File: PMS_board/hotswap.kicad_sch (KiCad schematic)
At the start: 28 parts, among them Q11 Q_NMOS_GDS, Q12 Q_NMOS_GDS, Q3 Q_NMOS_GDS, Q4 Q_NMOS_GDS, U12 LM74800QDRRRQ1, U7 LM74800QDRRRQ1

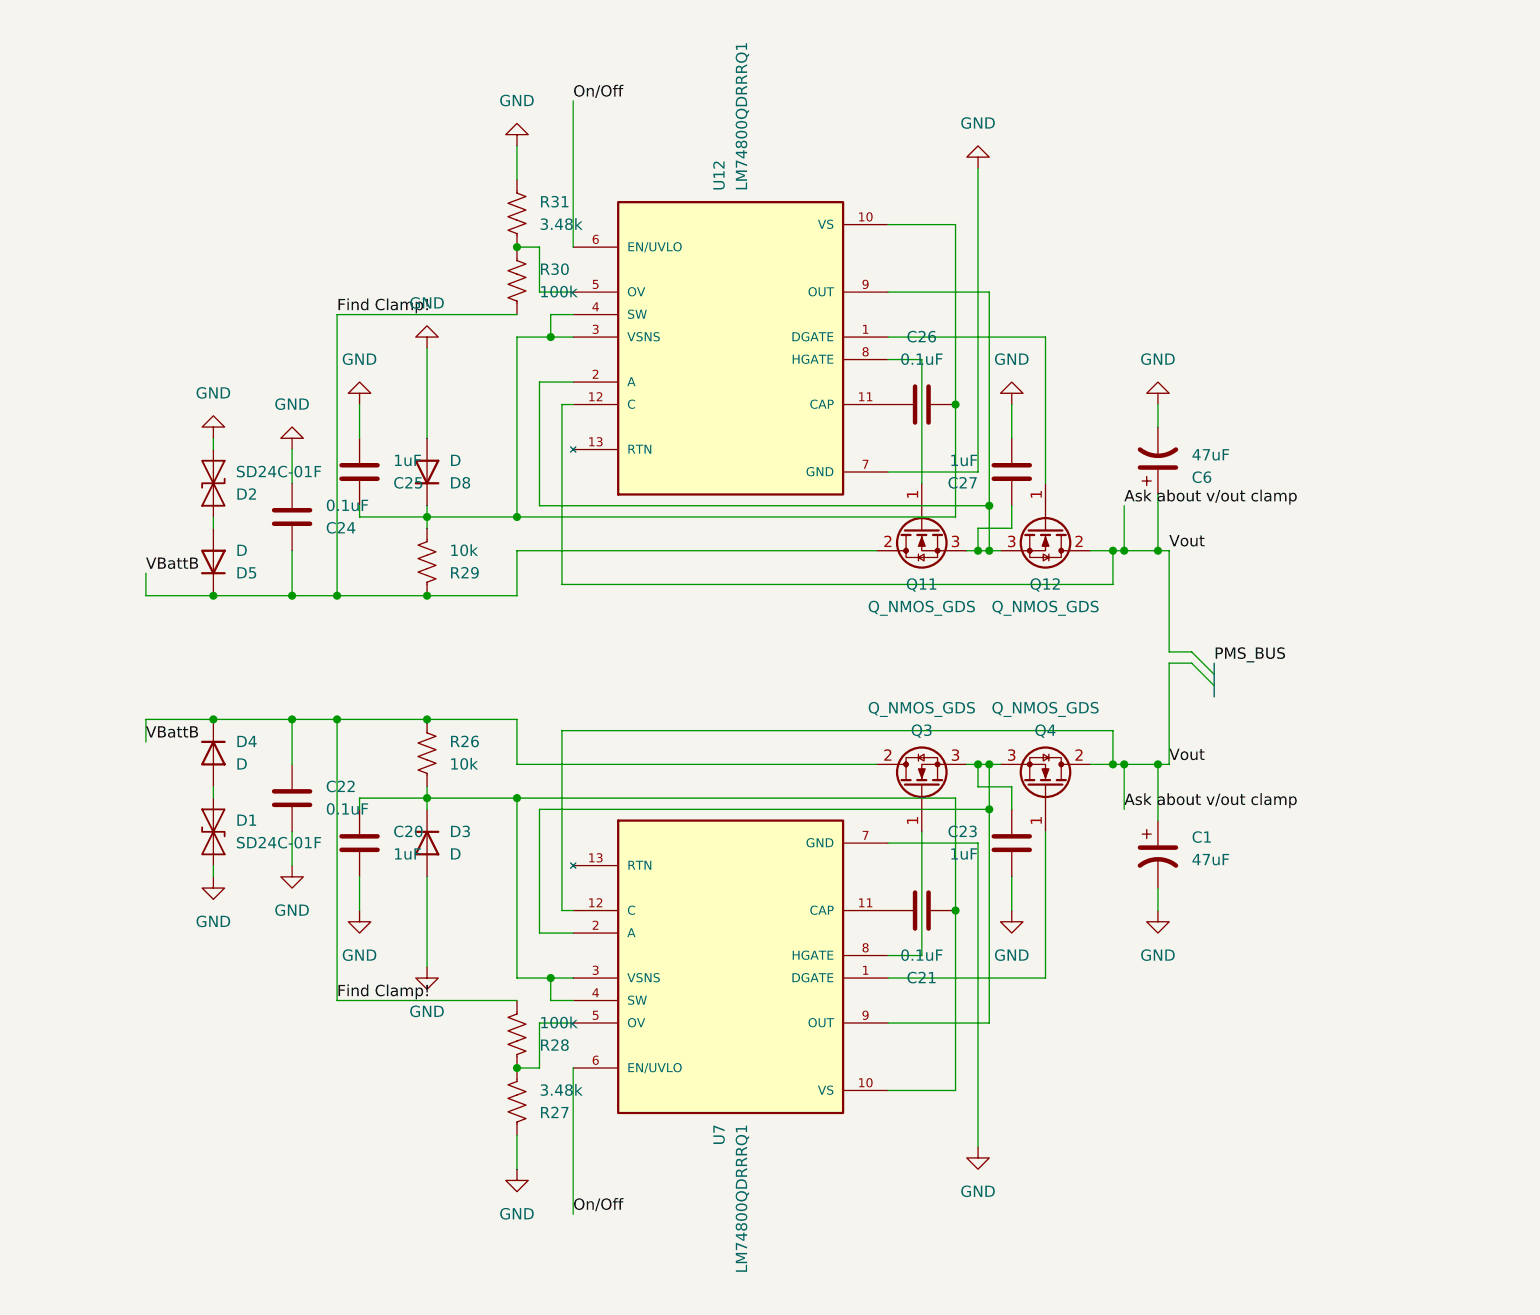
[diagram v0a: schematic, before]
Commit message: Fix Hotswap
I fixed hotswap, i think :)
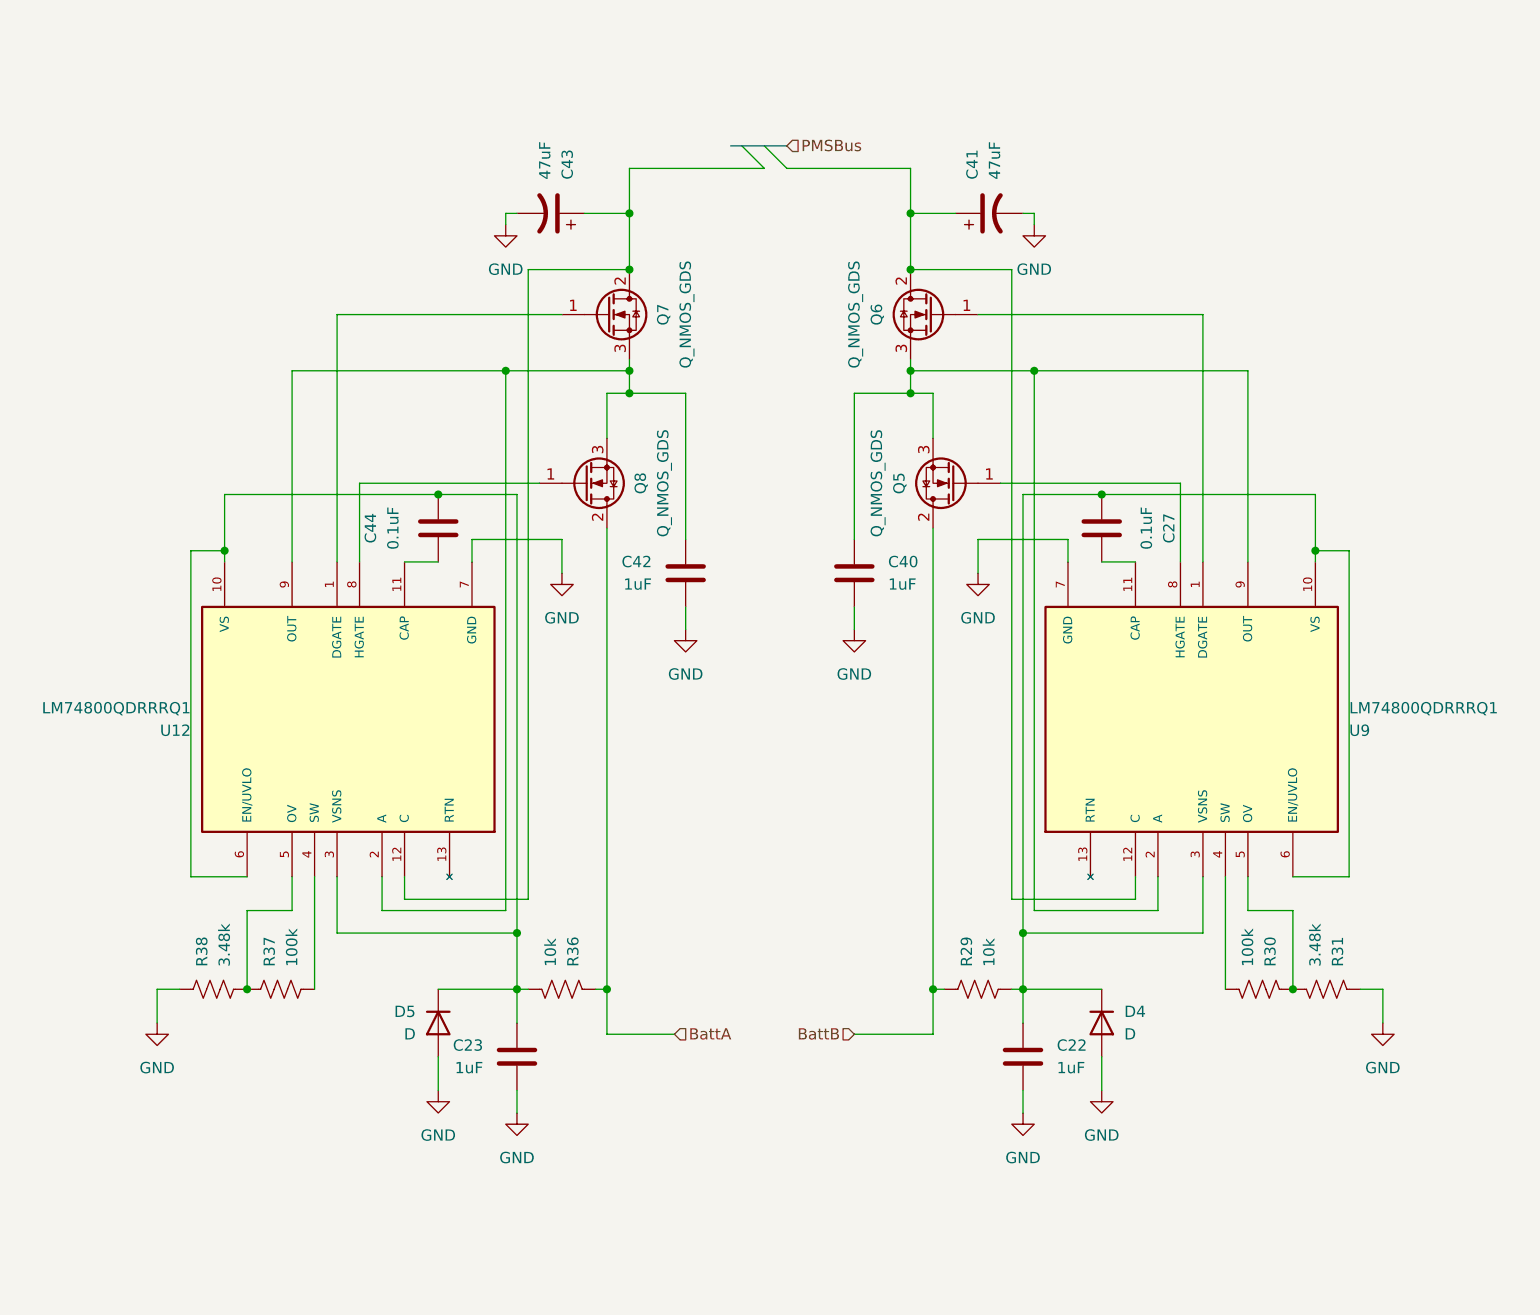
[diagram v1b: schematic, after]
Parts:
- removed C1, C6: 47uF, symbol Device:C_Polarized_US
- removed C20, C25: 1uF, symbol Device:C
- removed C21, C24, C26: 0.1uF, symbol Device:C
- removed D1, D2: SD24C-01F, Diode_SMD:D_SOD-323, symbol Diode:SD24C-01F
- removed D3, D8: D, symbol Device:D
- removed Q11, Q12, Q3, Q4: Q_NMOS_GDS, symbol Transistor_FET:Q_NMOS_GDS
- removed R26: 10k, symbol Device:R_US
- removed R27: 3.48k, symbol Device:R_US
- removed R28: 100k, symbol Device:R_US
- removed U7: LM74800QDRRRQ1, LM74800QDRRRQ1:IC_LM74800QDRRRQ1, symbol LM74800QDRRRQ1:LM74800QDRRRQ1
- added C40, C42: 1uF, symbol Device:C
- added C41, C43: 47uF, symbol Device:C_Polarized_US
- added C44: 0.1uF, symbol Device:C
- added Q5, Q6, Q7, Q8: Q_NMOS_GDS, symbol Transistor_FET:Q_NMOS_GDS
- added R36: 10k, symbol Device:R_US
- added R37: 100k, symbol Device:R_US
- added R38: 3.48k, symbol Device:R_US
- added U9: LM74800QDRRRQ1, LM74800QDRRRQ1:IC_LM74800QDRRRQ1, symbol LM74800QDRRRQ1:LM74800QDRRRQ1
- C22: value 0.1uF -> 1uF
- C27: value 1uF -> 0.1uF
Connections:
- net On/Off is gone; now on an unnamed net: U12.6 (EN/UVLO)
- net GND: now also C23.2, D4.2 (A), D5.2 (A), C40.2, C41.2, C42.2, C43.2, R38.1, U9.7 (GND); no longer C23.1, C27.1
- net at U12.11 (CAP): now also C44.1
- net at U12.10 (VS), U12.3 (VSNS): now also C23.1, D5.1 (K), C44.2, R36.2; no longer R29.2, U12.4 (SW)
- net at U12.2 (A), U12.9 (OUT): now also C42.1, Q7.3 (S), Q8.3 (S); no longer C27.2
- net at R30.1, R31.2: now also U9.5 (OV); no longer U12.5 (OV)
- net at U12.1 (DGATE): now also Q7.1 (G)
- net at U12.8 (HGATE): now also Q8.1 (G)
- net Ask about v/out clamp: no longer names the net of U12.12 (C)
- net Ask about v/out clamp: now also C43.1, Q7.2 (D)
- removed net Find Clamp!: C22.1, D4.1 (K), D5.1 (K), R29.1, R30.2
- new net: R37.1, R38.2, U12.5 (OV)
- new net: R37.2, U12.4 (SW)
- new net: R30.2, U9.4 (SW)
- new net: C27.1, U9.11 (CAP)
- new net: C22.1, C27.2, D4.1 (K), R29.2, U9.10 (VS), U9.3 (VSNS), U9.6 (EN/UVLO)
- new net: Q6.1 (G), U9.1 (DGATE)
- new net: C41.1, Q6.2 (D), U9.12 (C)
- new net: C40.1, Q5.3 (S), Q6.3 (S), U9.2 (A), U9.9 (OUT)
- new net: Q5.1 (G), U9.8 (HGATE)
- new net BattA: Q8.2 (D), R36.1
- new net BattB: Q5.2 (D), R29.1
